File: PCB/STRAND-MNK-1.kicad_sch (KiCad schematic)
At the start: 44 parts

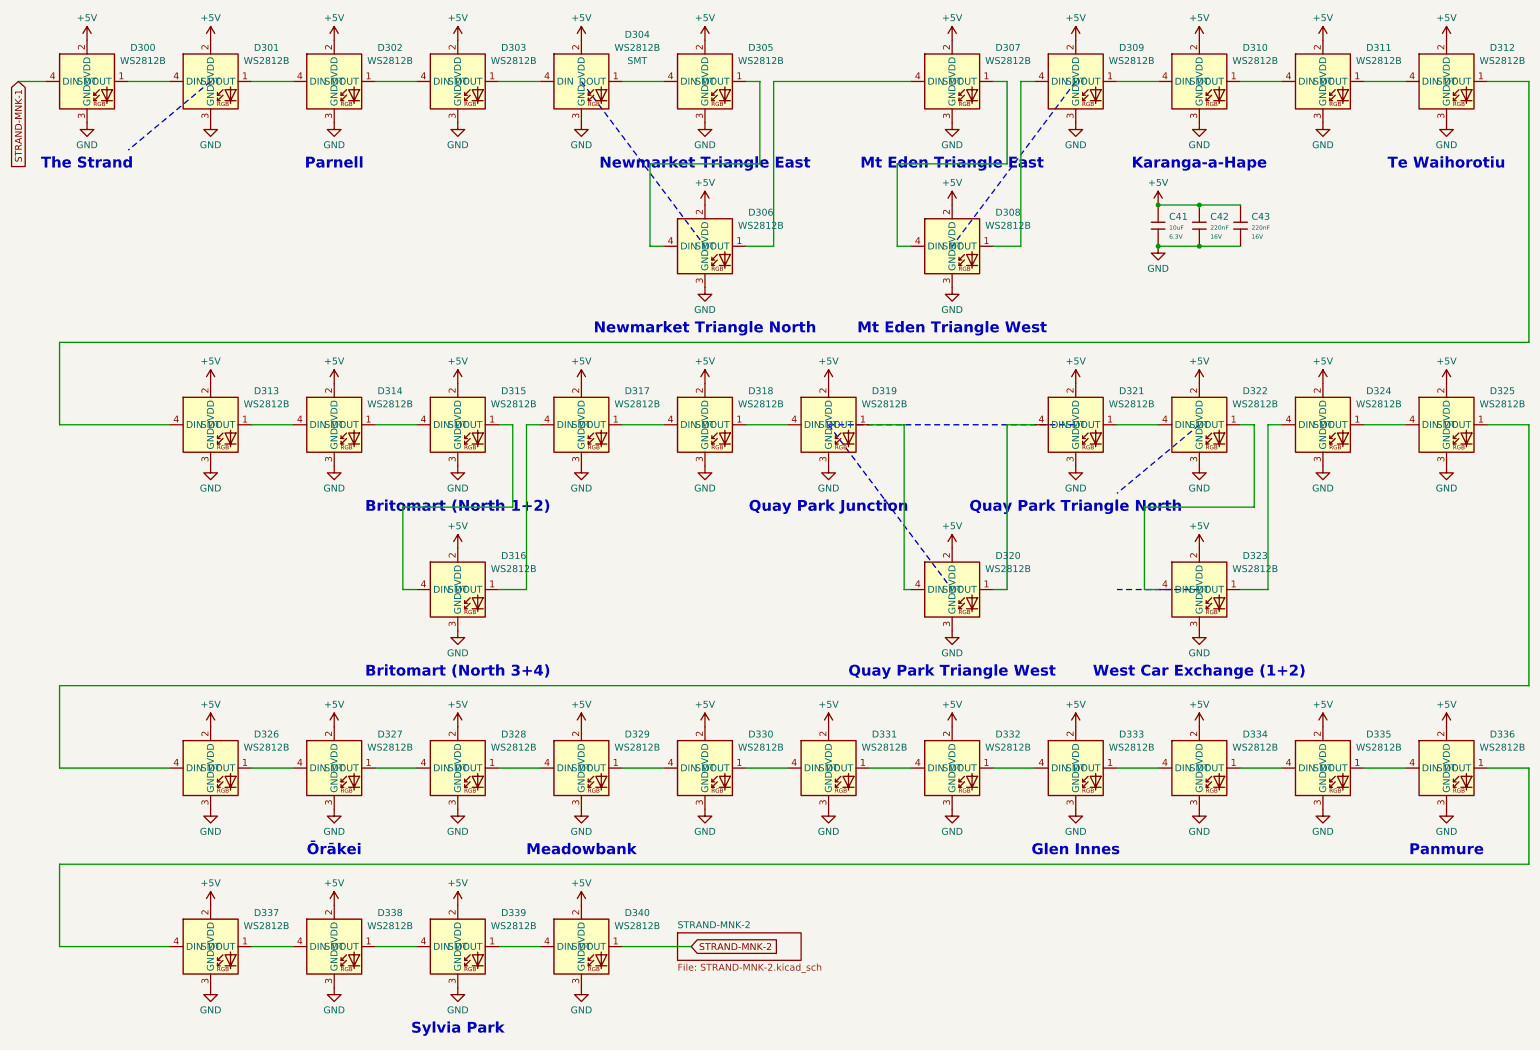
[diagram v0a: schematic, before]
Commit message: V1.1.0 PCB
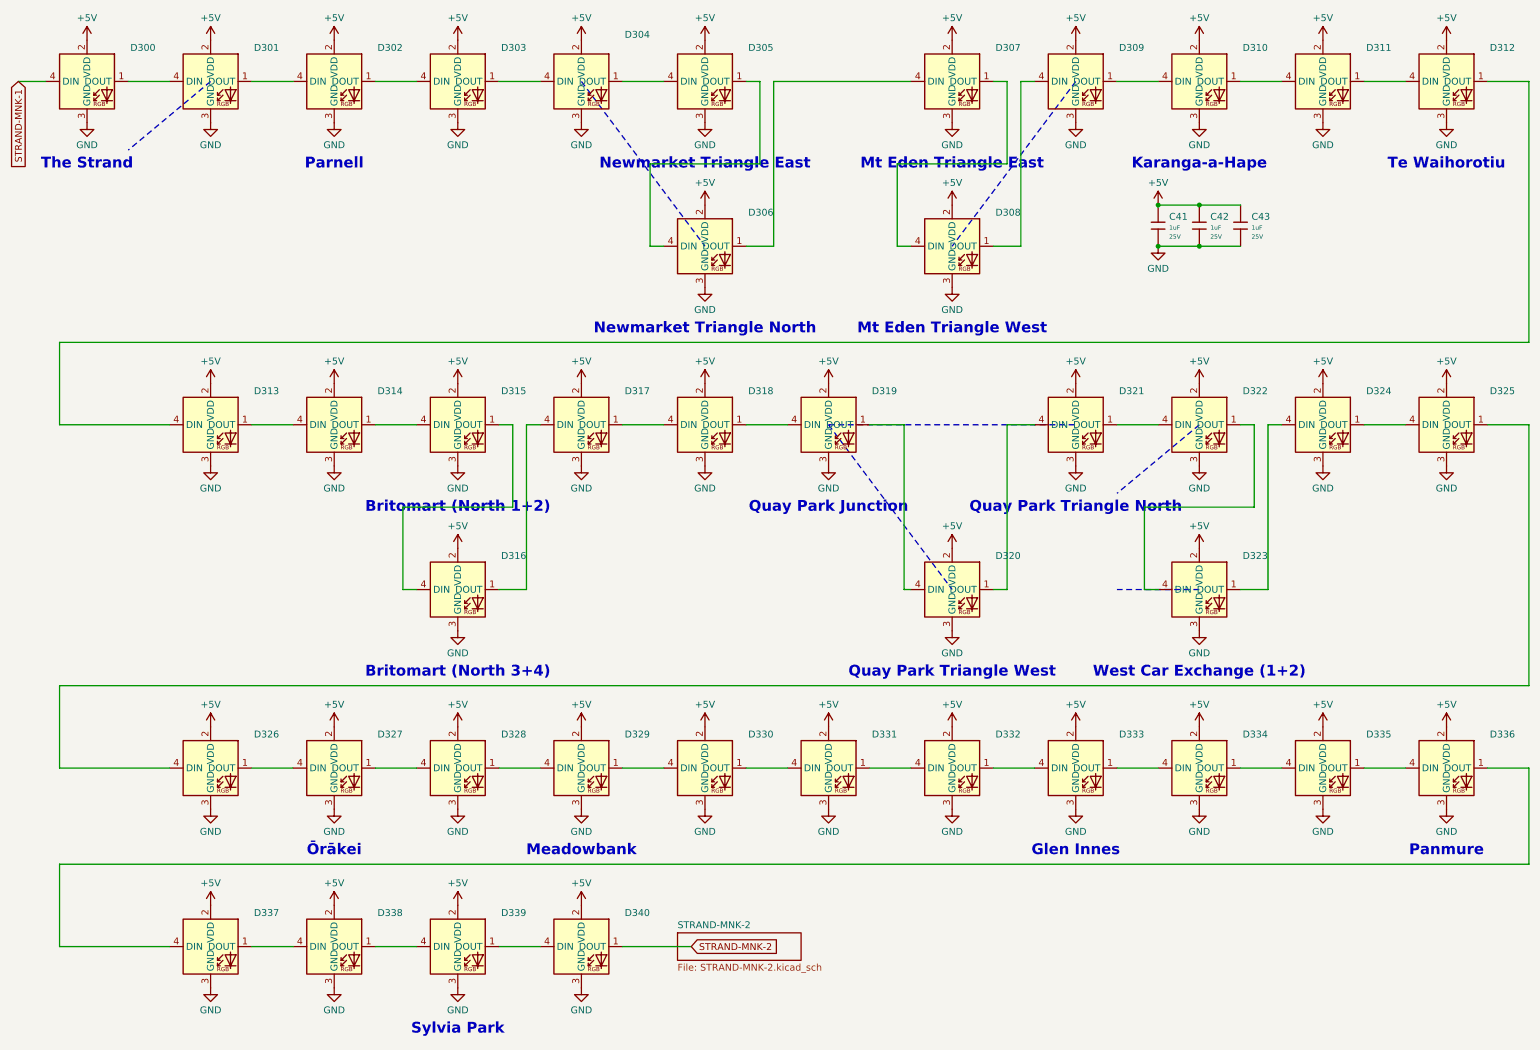
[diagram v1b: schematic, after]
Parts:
- C41: value 10uF -> 1uF; symbol PCM_JLCPCB-Capacitors:0402,10uF -> PCM_JLCPCB-Capacitors:0402,1uF; Capacitance 10uF -> 1uF; LCSC C15525 -> C52923; Part CL05A106MQ5NUNC -> CL05A105KA5NQNC; Price 0.007USD -> 0.006USD; Stock 1595146 -> 9606588; Tolerance ±20% -> ±10%; Voltage Rated 6.3V -> 25V
- C42, C43: value 220nF -> 1uF; symbol PCM_JLCPCB-Capacitors:0402,220nF -> PCM_JLCPCB-Capacitors:0402,1uF; Capacitance 220nF -> 1uF; LCSC C16772 -> C52923; Part CL05B224KO5NNNC -> CL05A105KA5NQNC; Price 0.008USD -> 0.006USD; Stock 351761 -> 9606588; Temperature Coefficient X7R -> X5R; Voltage Rated 16V -> 25V
- D300, D301, D302, D303, D304, D305, D306, D307, D308, D309, D310, D311, D312, D313, D314, D315, D316, D317, D318, D319, D320, D321, D322, D323, D324, D325, D326, D327, D328, D329, D330, D331, D332, D333, D334, D335, D336, D337, D338, D339, D340: value WS2812B -> XL-1615RGBC-WS2812B-S; LCSC C5349954 -> C41413180; Manufacturer XINGLIGHT -> (none); Part XL-1615RGBC-WS2812B -> (none); Process SMT -> (none)

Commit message: Update to meet OSHWA Certification
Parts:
- D300, D301, D302, D303, D304, D305, D306, D307, D308, D309, D310, D311, D312, D313, D314, D315, D316, D317, D318, D319, D320, D321, D322, D323, D324, D325, D326, D327, D328, D329, D330, D331, D332, D333, D334, D335, D336, D337, D338, D339, D340: Manufacturer (none) -> XINGLIGHT; Part (none) -> XL-1615RGBC-WS2812B-S
